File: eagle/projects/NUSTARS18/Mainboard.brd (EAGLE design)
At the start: 105 x 48 mm, 15 parts, among them IC1 7805T

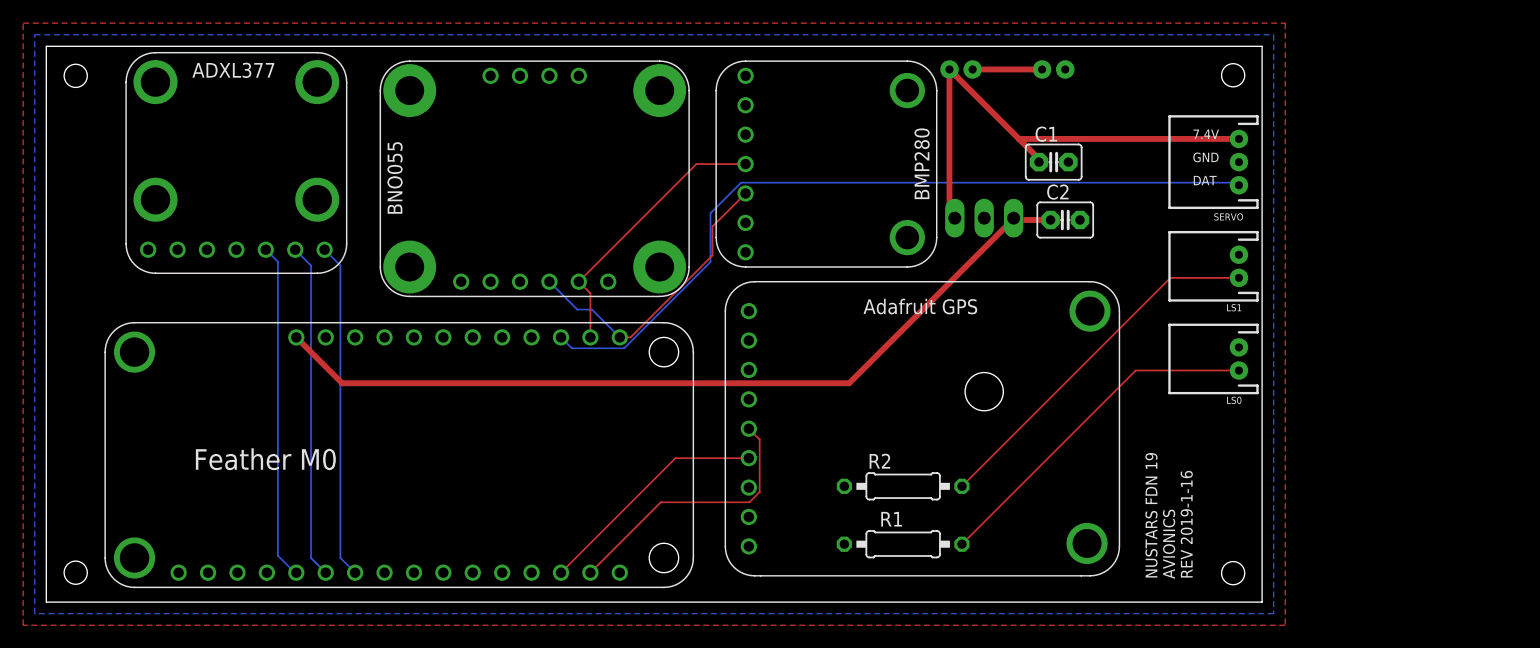
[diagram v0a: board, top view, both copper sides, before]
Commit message: Updated the board yet again
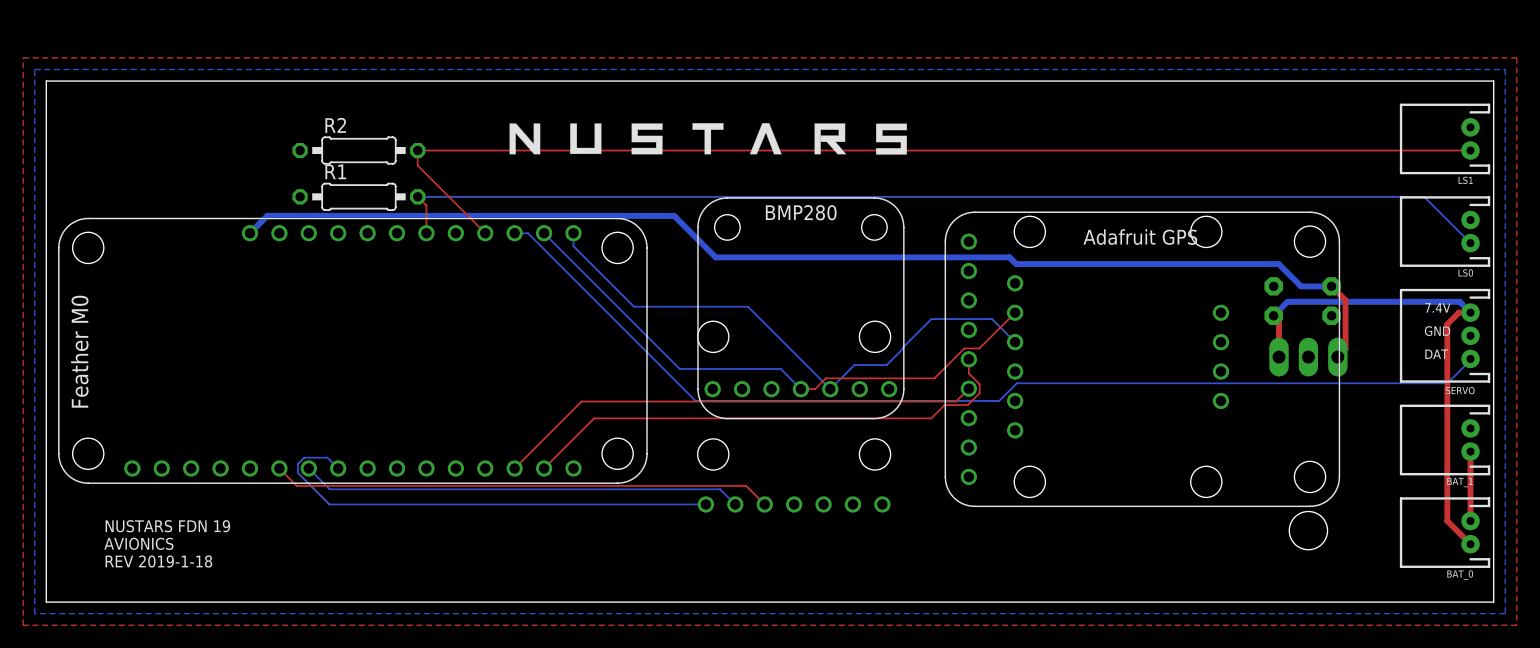
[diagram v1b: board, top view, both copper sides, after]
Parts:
- removed IC1: 7805T, linear:TO220H
- added IC0: 7805T, linear:TO220H
- C1, C2: value (none) -> 10uF
- moved U$3 70.7 mm to (74.1, 6.40), flipped to the bottom
- moved BAT_0 59.5 mm to (123.0, 6.00), flipped to the top, turned to 90 degrees
- moved R1 55.8 mm to (27.0, 35.0)
- moved R2 55.2 mm to (27.0, 39.0)
- moved U$5 52.7 mm to (92.6, 21.2), flipped to the bottom, turned to 90 degrees
- moved BAT_1 48.2 mm to (123.0, 14.0), flipped to the top, turned to 90 degrees
- moved U$2 30.9 mm to (56.3, 15.8), turned to 0 degrees
- moved SERVO 25.0 mm to (123.0, 23.0)
- moved C2 24.0 mm to (111.0, 26.0), flipped to the bottom, turned to 270 degrees
- moved LS0 22.8 mm to (123.0, 32.0)
- moved LS1 22.8 mm to (123.0, 40.0)
- moved C1 22.5 mm to (106.0, 26.0), flipped to the bottom, turned to 90 degrees
- moved U$4 19.9 mm to (94.7, 21.0)
- moved U$1 9.85 mm to (16.3, 21.7)
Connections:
- removed net 5V_REG: C2.1, IC1.3, U$1.BAT
- new net 5V_REG_M0: C2.1, IC0.3, U$1.BAT
- net ADXL_X: now also U$1.A3; no longer U$1.A2
- net ADXL_Y: now also U$1.A2; no longer U$1.A1
- net ADXL_Z: now also U$1.A1; no longer U$1.A0
- net GND: now also IC0.2; no longer IC1.2
- net LS0_D: now also U$1.10
- net LS1_D: now also U$1.6
- net V_BAT: now also IC0.1; no longer IC1.1
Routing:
- net 5V_REG_M0: track 0.00 -> 103.4 mm
- net 5V_REG: track 72.8 -> 0.00 mm
- net LS1_D: track 31.4 -> 100.5 mm
- net LS0_D: track 30.1 -> 96.0 mm
- net CLK: track 23.8 -> 49.0 mm
- net D_SERVO: track 67.4 -> 90.1 mm
- net DAT: track 25.5 -> 47.8 mm
- net RX: track 20.3 -> 42.1 mm
- net TX: track 23.4 -> 43.6 mm
- net ADXL_Z: track 29.1 -> 43.2 mm
- net ADXL_X: track 29.0 -> 41.2 mm
- net ADXL_Y: track 29.0 -> 38.1 mm
- net V_BAT: track 43.2 -> 43.9 mm
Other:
- board size 105 x 48 mm -> 125 x 45 mm
- board text added: "NUSTARS FDN 19 AVIONICS REV 2019-1-18"
- board text removed: "+3.7V"
- board text removed: "NUSTARS FDN 19 AVIONICS REV 2019-1-16"
